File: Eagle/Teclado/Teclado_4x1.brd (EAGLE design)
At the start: 55 x 25 mm, 6 parts, among them J1 ZCN_5PIN, P1 BOTON_TECLADO, P2 BOTON_TECLADO, P3 BOTON_TECLADO, P4 BOTON_TECLADO

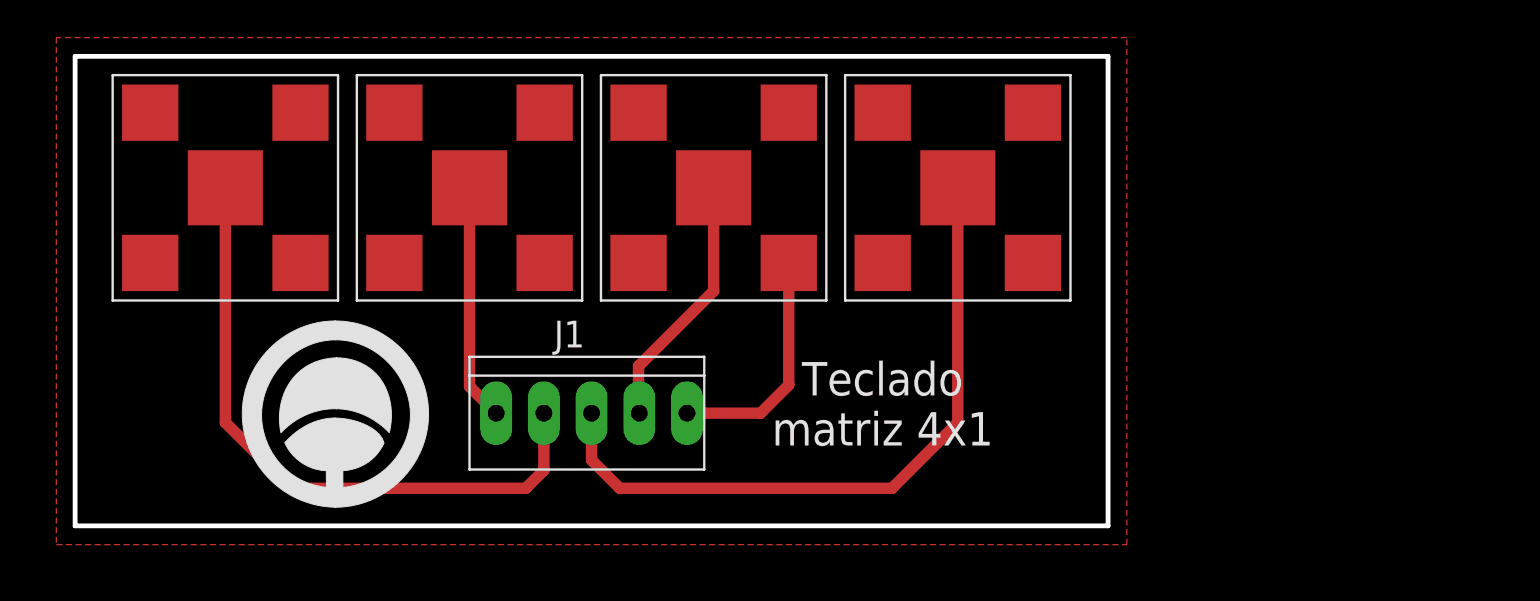
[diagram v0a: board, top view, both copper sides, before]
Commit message: Terminado PCB teclado
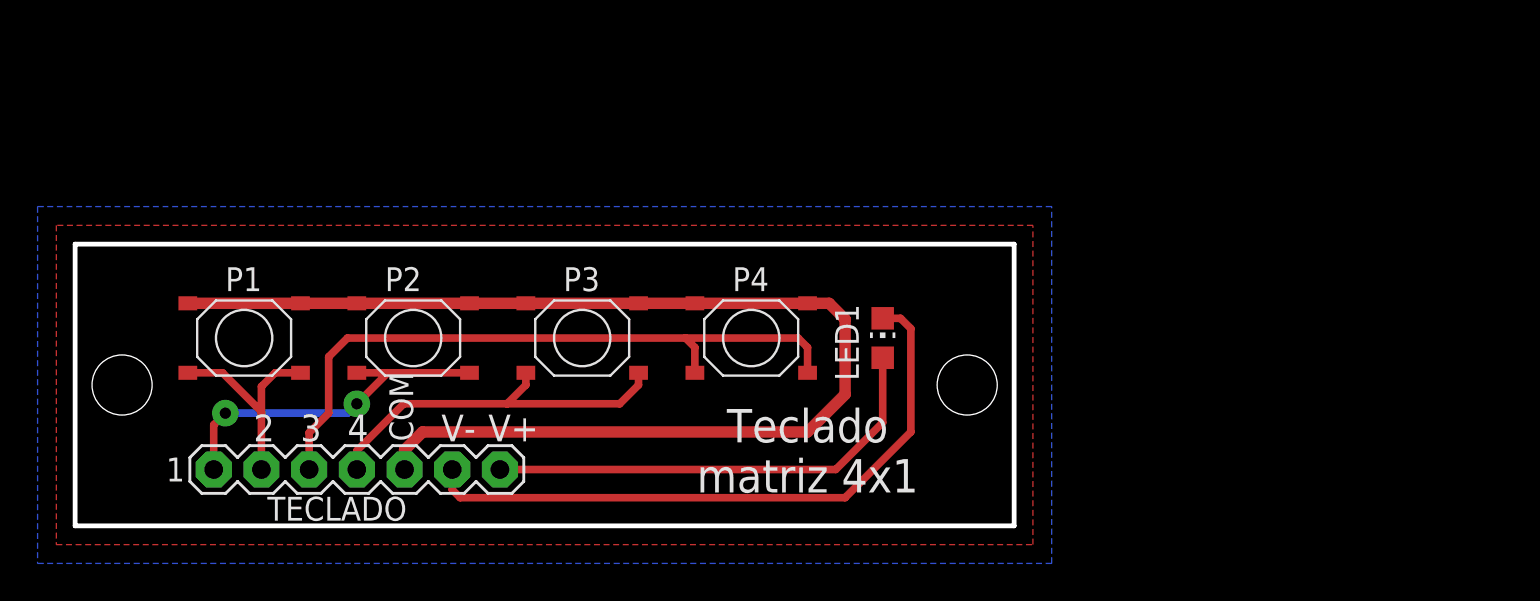
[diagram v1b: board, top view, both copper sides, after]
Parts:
- removed J1: ZCN_5PIN, Circuitos-Creativos-Conectores:ZCN_5PIN_2.54MM
- added LED1: (no value), led:CHIP-LED0805
- added TECLADO: (no value), con-lstb:MA07-1
- P1, P2, P3, P4: value BOTON_TECLADO -> PULSADOR5.2X5.2; device Circuitos-Creativos-Conectores:BOTON_TECLADO -> Circuitos-Creativos-Conectores:SMT_5.2X5.2MM
- moved U$1 25.2 mm to (39.0, 7.50), flipped to the bottom
- moved P4 13.6 mm to (36.0, 10.0)
- moved P3 10.6 mm to (27.0, 10.0)
- moved P2 8.54 mm to (18.0, 10.0)
- moved P1 8.06 mm to (9.00, 10.0)
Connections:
- new net N$1: LED1.C, TECLADO.6
- new net N$2: LED1.A, TECLADO.7
- net C1: now also TECLADO.5; no longer J1.5, P1.3, P1.4, P2.3, P2.4, P3.3, P3.4, P4.3, P4.4
- net F1: now also P1.3, P1.4, TECLADO.2; no longer J1.2, P1.5
- net F2: now also P2.3, P2.4, TECLADO.1; no longer J1.1, P2.5
- net F3: now also P3.3, P3.4, TECLADO.4; no longer J1.4, P3.5
- net F4: now also P4.3, P4.4, TECLADO.3; no longer J1.3, P4.5
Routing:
- net C1: track 12.5 -> 65.1 mm
- net N$1: track 0.00 -> 34.4 mm
- net N$2: track 0.00 -> 24.9 mm
- net F1: track 34.3 -> 11.6 mm
- net F3: track 13.7 -> 20.2 mm
- net F2: track 12.6 -> 18.8 mm, vias 0 -> 2
- net F4: track 36.6 -> 36.0 mm
- added copper zone on layer 16, net C1
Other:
- board size 55 x 25 mm -> 50 x 15 mm
- board text added: "2"
- board text added: "3"
- board text added: "4"
- board text added: "COM"
- board text added: "V+"
- board text added: "V-"

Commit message: Cambio solicitado por Segcontrol SAS
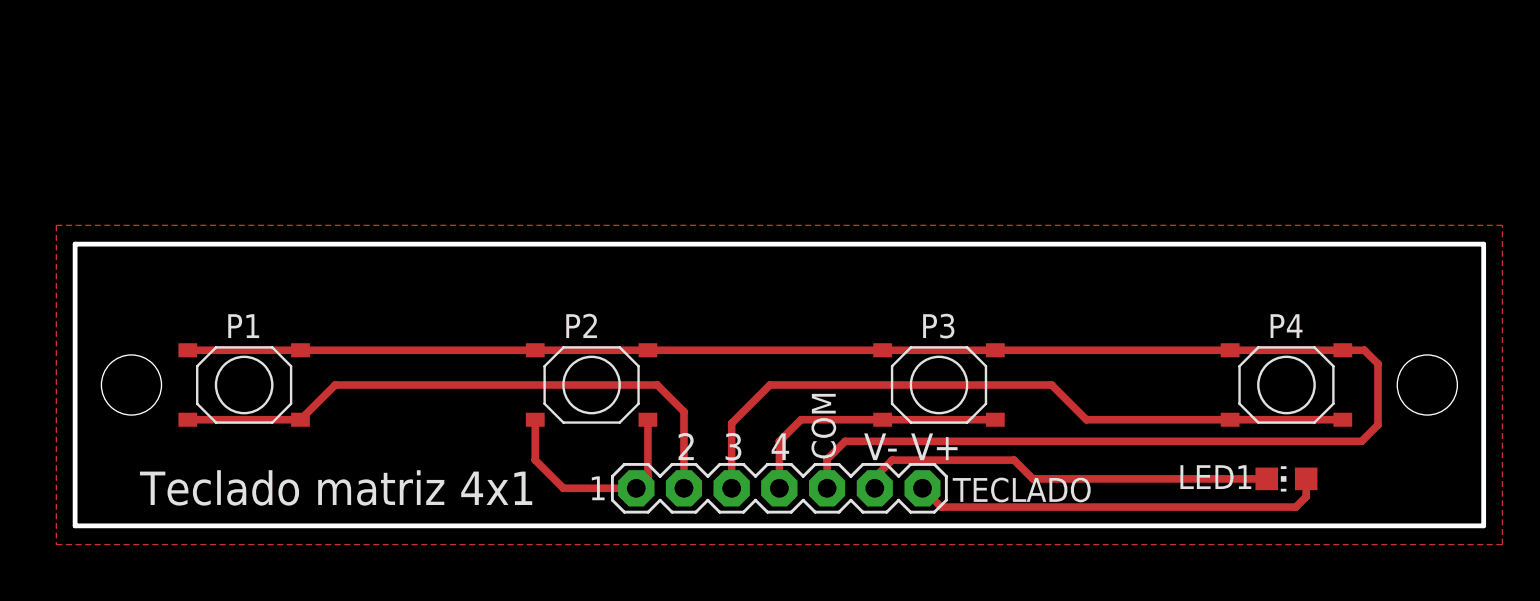
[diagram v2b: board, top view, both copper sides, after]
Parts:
- LED1: value (none) -> verde
- moved P4 28.6 mm to (64.5, 7.50)
- moved LED1 22.8 mm to (64.5, 2.50), turned to 90 degrees
- moved TECLADO 22.5 mm to (37.5, 2.00)
- moved P3 19.2 mm to (46.0, 7.50)
- moved P2 9.82 mm to (27.5, 7.50)
- moved P1 2.50 mm to (9.00, 7.50)
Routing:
- net C1: track 65.1 -> 98.6 mm
- net F1: track 11.6 -> 31.9 mm
- net N$1: track 34.4 -> 22.2 mm
- net F2: track 18.8 -> 12.1 mm, vias 2 -> 0
- net F3: track 20.2 -> 14.5 mm
- net N$2: track 24.9 -> 22.0 mm
- net F4: track 36.0 -> 37.6 mm
- removed copper zone on layer 16, net C1
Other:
- board size 50 x 15 mm -> 75 x 15 mm
